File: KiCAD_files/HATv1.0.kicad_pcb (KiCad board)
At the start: 4 copper layers, 65 x 56.5 mm, 44 parts, among them J1 Conn_Coaxial, J2 Conn_Coaxial, J3 USB_B_Micro, J4 raspberrypi_hat_OX40HAT, J5 Conn_01x04_Male, J6 Conn_01x06_Male, J7 Conn_01x02_Male, U1 mosaic-X5, U2 LD1117AS33TR, U3 SN74AVC4T245PW, U4 SN74LVC1G126DRLR

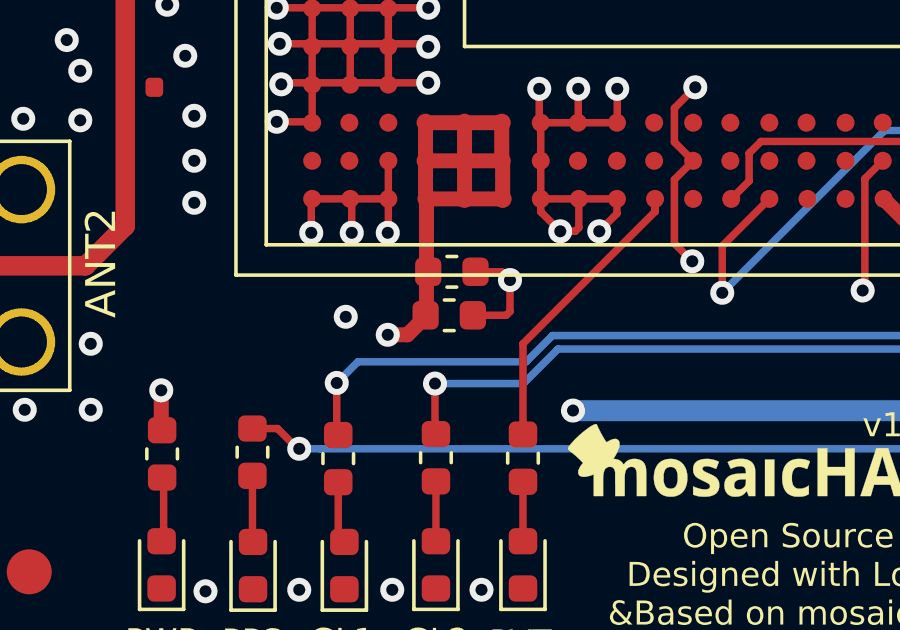
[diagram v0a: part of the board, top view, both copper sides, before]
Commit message: update project
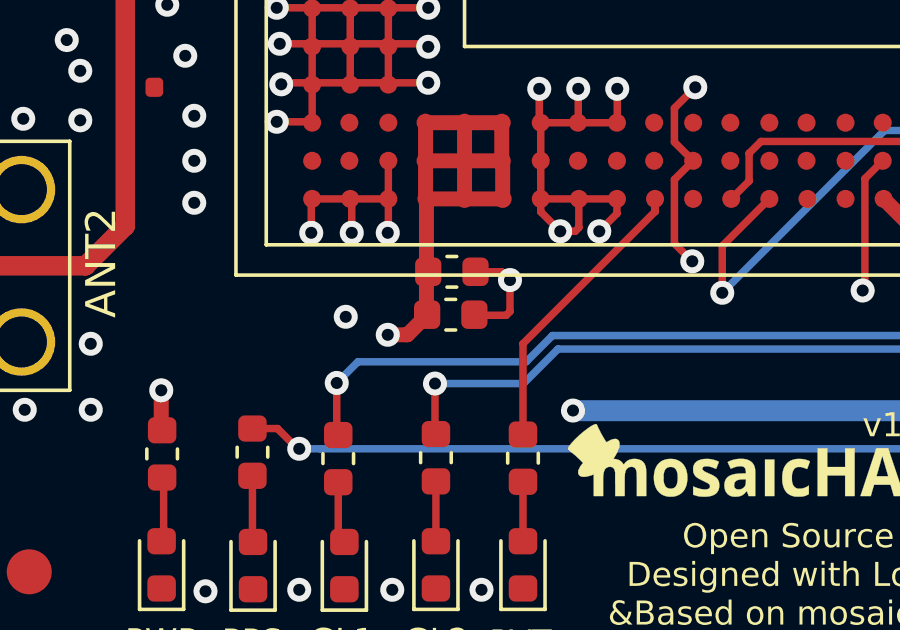
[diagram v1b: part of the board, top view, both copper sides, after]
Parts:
- removed the C6 at (143.7, 65.8)
- added C7: un-assembled, Capacitor_SMD:C_0603_1608Metric, F.Cu at (143.8, 65.8)
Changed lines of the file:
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@@
     (add_net /USB_P)
+  )
+  (module Capacitor_SMD:C_0603_1608Metric (layer F.Cu)
+    (at 143.75 65.83)
+    (descr "Capacitor SMD 0603 (1608 Metric), square (rectangular) end terminal, IPC_7351 nominal, (Body size source: http://www.tortai-tech.com/upload/download/2011102023233369053.pdf), generated with kicad-footprint-generator")
+    (tags capacitor)
+    (attr smd)
+    (fp_text reference C7 (at 0 -1.43) (layer F.SilkS) hide
+      (effects (font (size 1 1) (thickness 0.15)))
+    )
+    (fp_text value un-assembled (at 0 1.43) (layer F.Fab)
+      (effects (font (size 1 1) (thickness 0.15)))
+    )
+    (fp_line (start 1.48 0.73) (end -1.48 0.73) (layer F.CrtYd) (width 0.05))
+    (fp_line (start 1.48 -0.73) (end 1.48 0.73) (layer F.CrtYd) (width 0.05))
+    (fp_line (start -1.48 -0.73) (end 1.48 -0.73) (layer F.CrtYd) (width 0.05))
+    (fp_line (start -1.48 0.73) (end -1.48 -0.73) (layer F.CrtYd) (width 0.05))
+    (fp_line (start -0.162779 0.51) (end 0.162779 0.51) (layer F.SilkS) (width 0.12))
+    (fp_line (start -0.162779 -0.51) (end 0.162779 -0.51) (layer F.SilkS) (width 0.12))
+    (fp_line (start 0.8 0.4) (end -0.8 0.4) (layer F.Fab) (width 0.1))
+    (fp_line (start 0.8 -0.4) (end 0.8 0.4) (layer F.Fab) (width 0.1))
+    (fp_line (start -0.8 -0.4) (end 0.8 -0.4) (layer F.Fab) (width 0.1))
+    (fp_line (start -0.8 0.4) (end -0.8 -0.4) (layer F.Fab) (width 0.1))
+    (fp_text user %R (at 0 0) (layer F.Fab)
+      (effects (font (size 0.4 0.4) (thickness 0.06)))
+    )
+    (pad 2 smd roundrect (at 0.7875 0) (size 0.875 0.95) (layers F.Cu F.Paste F.Mask) (roundrect_rratio 0.25)
+      (net 1 GND))
+    (pad 1 smd roundrect (at -0.7875 0) (size 0.875 0.95) (layers F.Cu F.Paste F.Mask) (roundrect_rratio 0.25)
+      (net 2 +3V3))
   )
   (module openHW_small (layer F.Cu)
@@
     )
   )
-  (module Capacitor_SMD:C_0603_1608Metric (layer F.Cu)
-    (at 143.7 65.85)
-    (descr "Capacitor SMD 0603 (1608 Metric), square (rectangular) end terminal, IPC_7351 nominal, (Body size source: http://www.tortai-tech.com/upload/download/2011102023233369053.pdf), generated with kicad-footprint-generator")
-    (tags capacitor)
-    (attr smd)
-    (fp_text reference C6 (at 0 -1.43) (layer F.SilkS) hide
-      (effects (font (size 1 1) (thickness 0.15)))
-    )
-    (fp_text value 10uF (at 0 1.43) (layer F.Fab)
-      (effects (font (size 1 1) (thickness 0.15)))
-    )
-    (fp_line (start -0.8 0.4) (end -0.8 -0.4) (layer F.Fab) (width 0.1))
-    (fp_line (start -0.8 -0.4) (end 0.8 -0.4) (layer F.Fab) (width 0.1))
-    (fp_line (start 0.8 -0.4) (end 0.8 0.4) (layer F.Fab) (width 0.1))
-    (fp_line (start 0.8 0.4) (end -0.8 0.4) (layer F.Fab) (width 0.1))
-    (fp_line (start -0.162779 -0.51) (end 0.162779 -0.51) (layer F.SilkS) (width 0.12))
-    (fp_line (start -0.162779 0.51) (end 0.162779 0.51) (layer F.SilkS) (width 0.12))
-    (fp_line (start -1.48 0.73) (end -1.48 -0.73) (layer F.CrtYd) (width 0.05))
-    (fp_line (start -1.48 -0.73) (end 1.48 -0.73) (layer F.CrtYd) (width 0.05))
-    (fp_line (start 1.48 -0.73) (end 1.48 0.73) (layer F.CrtYd) (width 0.05))
-    (fp_line (start 1.48 0.73) (end -1.48 0.73) (layer F.CrtYd) (width 0.05))
-    (fp_text user %R (at 0 0) (layer F.Fab)
-      (effects (font (size 0.4 0.4) (thickness 0.06)))
-    )
-    (pad 1 smd roundrect (at -0.7875 0) (size 0.875 0.95) (layers F.Cu F.Paste F.Mask) (roundrect_rratio 0.25)
-      (net 2 +3V3))
-    (pad 2 smd roundrect (at 0.7875 0) (size 0.875 0.95) (layers F.Cu F.Paste F.Mask) (roundrect_rratio 0.25)
-      (net 1 GND))
-  )
   (module Fiducial:Fiducial_1.5mm_Mask3mm (layer F.Cu)
